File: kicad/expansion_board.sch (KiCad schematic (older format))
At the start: 5 parts

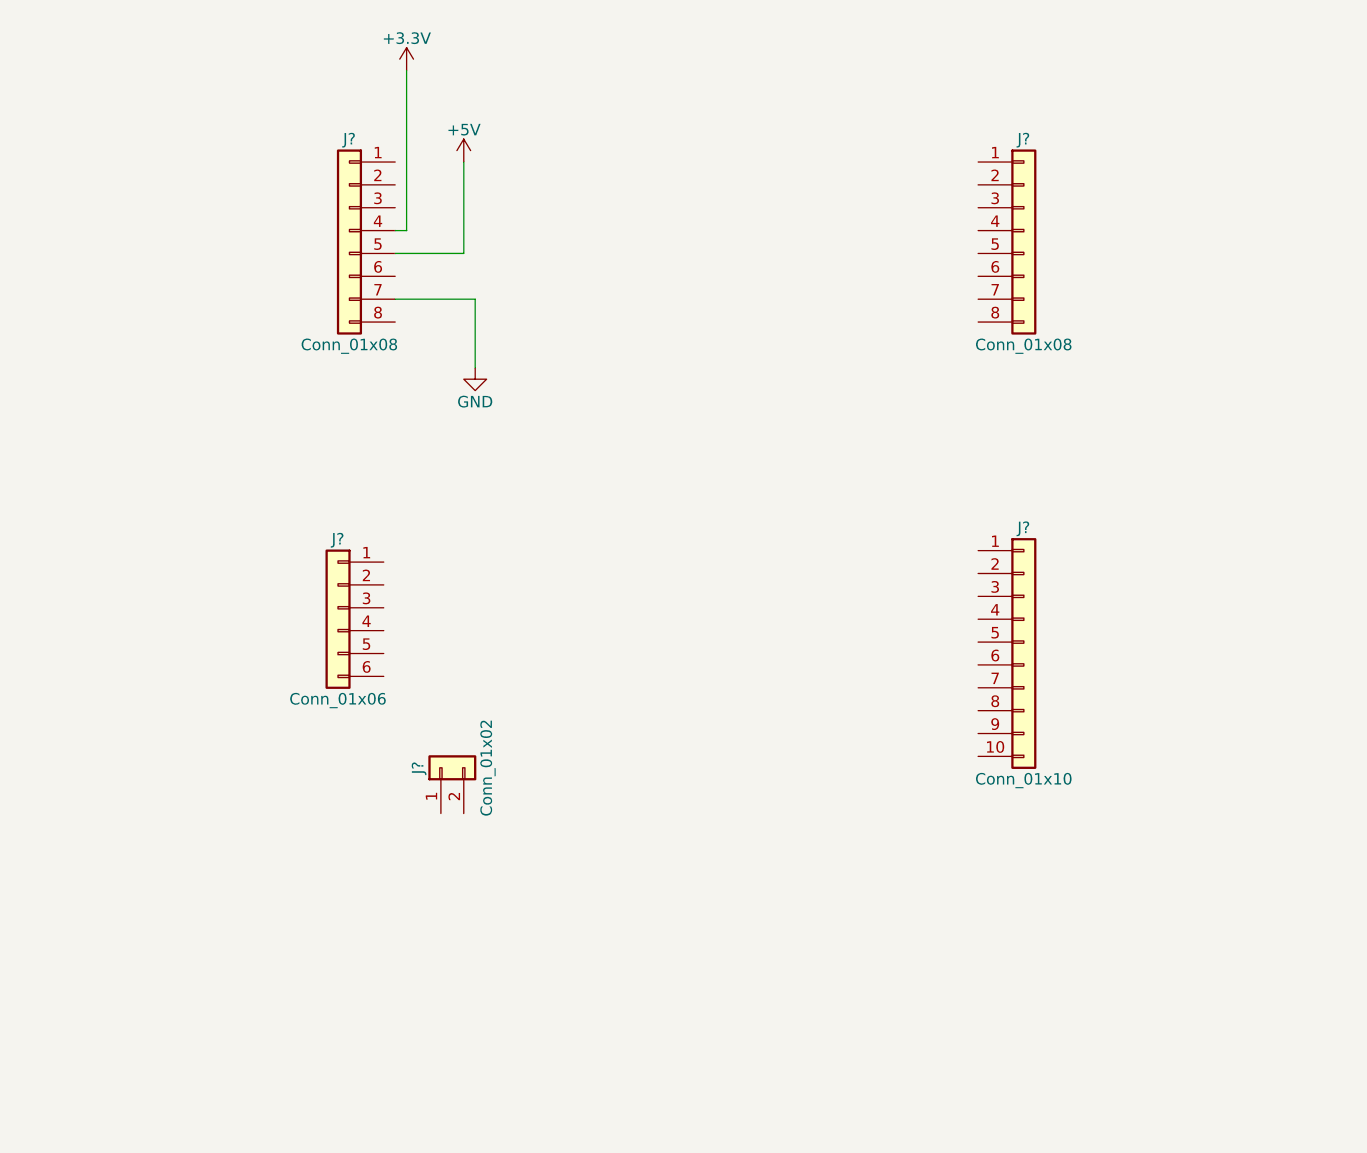
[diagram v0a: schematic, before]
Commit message: update
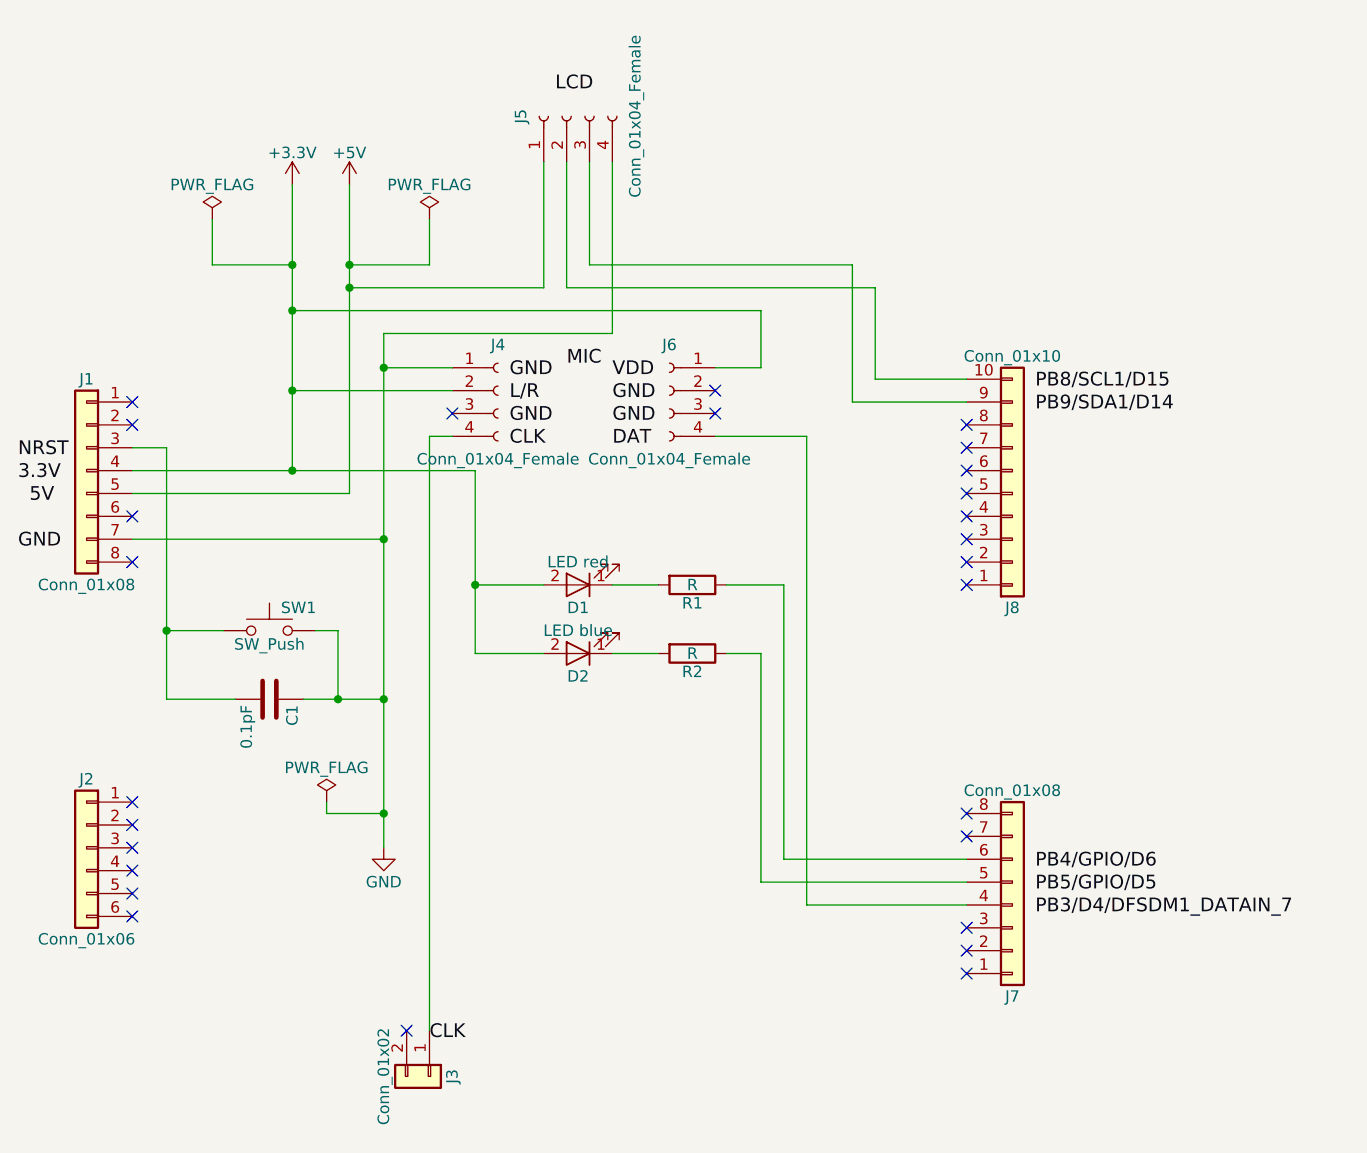
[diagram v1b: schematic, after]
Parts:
- removed J?: Conn_01x08, symbol Conn_01x08
- added C1: 0.1pF, symbol C
- added D1: LED red, symbol LED
- added D2: LED blue, symbol LED
- added J4, J5, J6: Conn_01x04_Female, symbol Conn_01x04_Female
- added J7: Conn_01x08, symbol Conn_01x08
- added R1, R2: R, symbol R
- added SW1: SW_Push, symbol SW_Push
- gave numbers to parts that had none: 4
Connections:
- net +3V3: now also D1.2 (A), D2.2 (A), J4.2 (Pin_2), J6.1 (Pin_1)
- net +5V: now also J5.1 (Pin_1)
- net GND: now also C1.1, J4.1 (Pin_1), J5.4 (Pin_4), SW1.2
- net at J1.3 (Pin_3): now also C1.2, SW1.1
- net at J8.10 (Pin_10): now also J5.2 (Pin_2)
- net at J8.9 (Pin_9): now also J5.3 (Pin_3)
- net at J3.1 (Pin_1): now also J4.4 (Pin_4)
- new net: J6.4 (Pin_4), J7.4 (Pin_4)
- new net: D1.1 (K), R1.2
- new net: D2.1 (K), R2.2
- new net: J7.6 (Pin_6), R1.1
- new net: J7.5 (Pin_5), R2.1
- no-connect marks 0 -> 27
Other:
- moved on the sheet: J1, J2, J3, J8
